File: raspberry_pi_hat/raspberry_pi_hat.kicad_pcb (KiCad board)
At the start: 2 copper layers, 100.5 x 49 mm, 18 parts, among them IC1 LD1117v33, J1 Screw_Terminal_01x02, J10 LED_status, J2 LCD_screeen, J8 GPIO, J9 Switches, U1 NRF24L01P

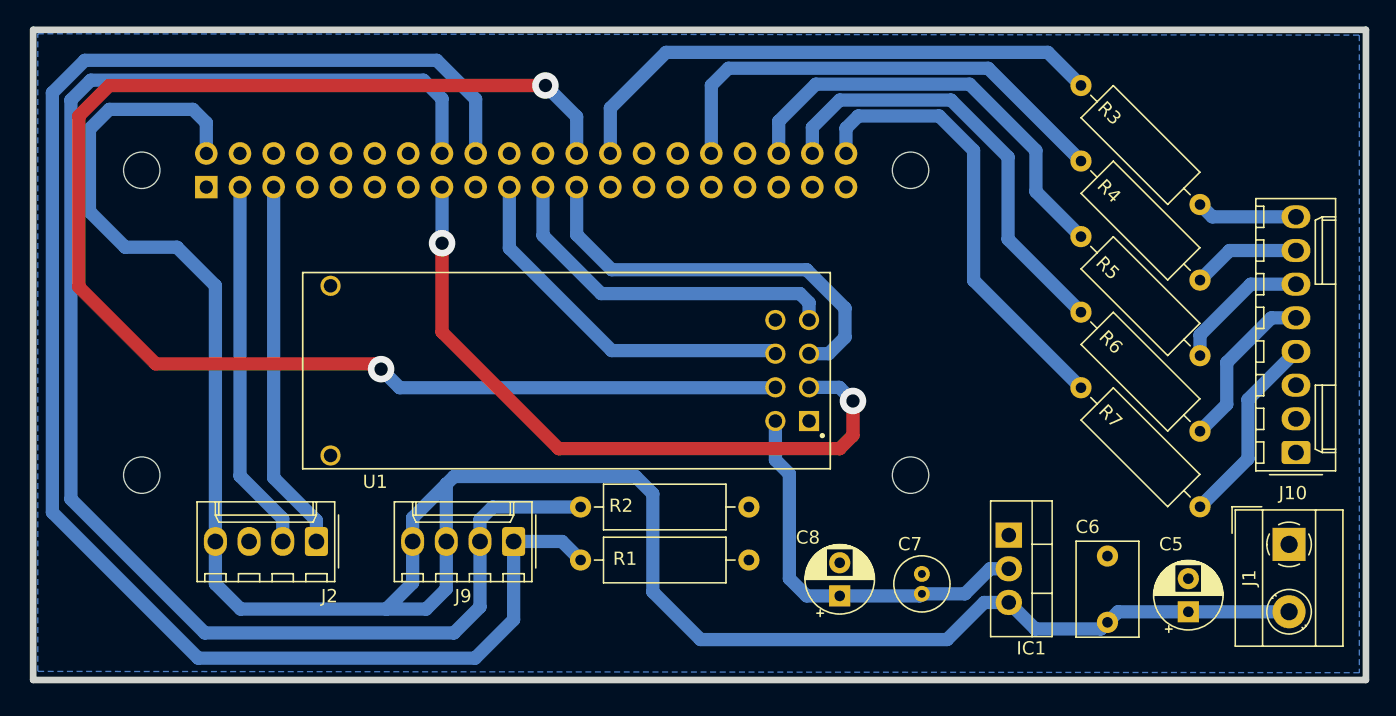
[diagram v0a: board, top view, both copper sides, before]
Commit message: improved final version
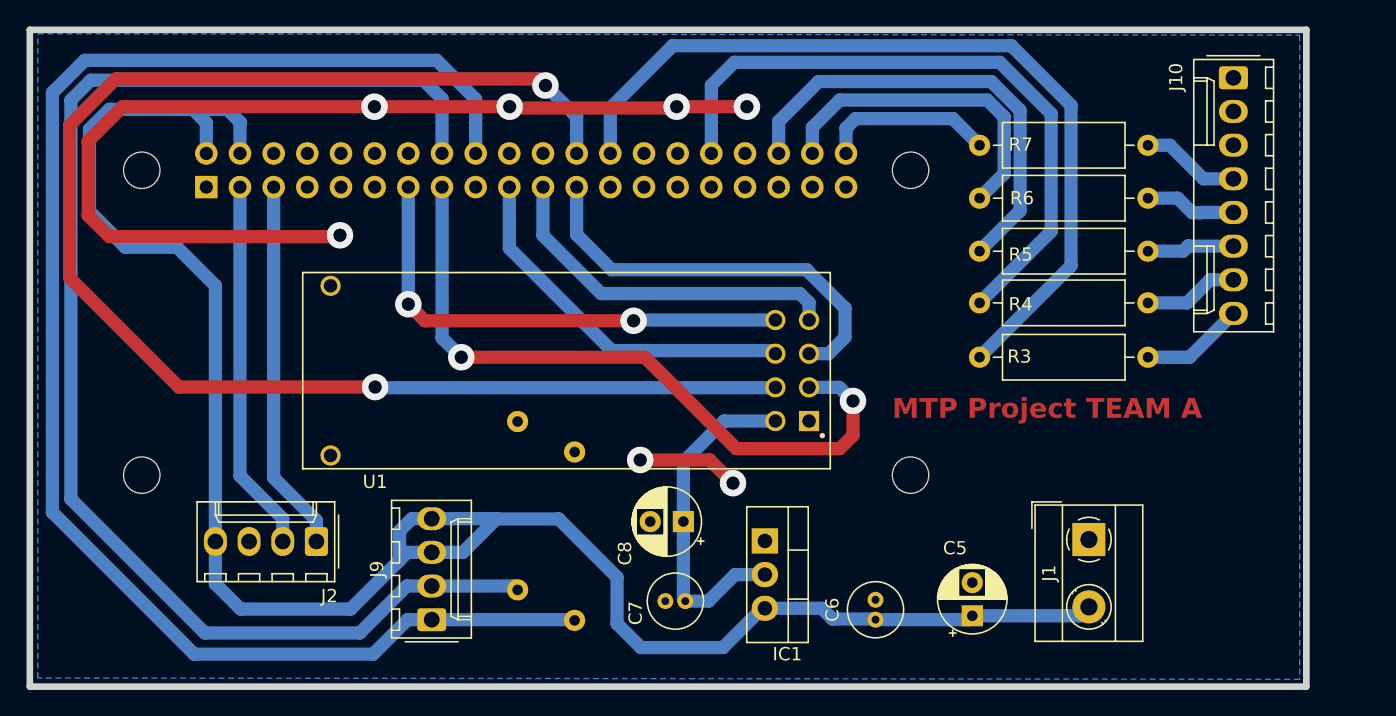
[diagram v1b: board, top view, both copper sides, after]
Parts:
- C6: footprint Capacitor_THT:C_Rect_L7.0mm_W4.5mm_P5.00mm -> Capacitor_THT:C_Radial_D4.0mm_H5.0mm_P1.50mm
- R1, R2: moved to B.Cu
- moved J10 28.7 mm to (205.5, 110.4), turned to -90 degrees
- moved R3 21.9 mm to (186.4, 131.5), turned to 0 degrees
- moved R7 19.8 mm to (186.4, 115.5), turned to 0 degrees
- moved IC1 18.4 mm to (170.2, 145.4)
- moved C7 17.9 mm to (164.2, 149.9), turned to 180 degrees
- moved C6 17.5 mm to (178.5, 151.3)
- moved C5 16.3 mm to (185.8, 151.0)
- moved J1 15.1 mm to (194.6, 145.3)
- moved R4 13.2 mm to (186.4, 127.4), turned to 0 degrees
- moved C8 13.1 mm to (164.0, 143.9), turned to 180 degrees
- moved R6 11.5 mm to (186.4, 119.5), turned to 0 degrees
- moved J9 8.54 mm to (145.0, 151.3), turned to 90 degrees
- moved R2 7.85 mm to (151.5, 149.1), turned to 90 degrees
- moved R5 7.73 mm to (186.4, 123.5), turned to 0 degrees
- moved R1 4.57 mm to (155.8, 151.3), turned to 90 degrees
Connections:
- U1 pad 8: unconnected-(U1-~{IRQ}-Pad8) -> /GPIO27
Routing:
- net GND: track 0.00 -> 83.9 mm, vias 0 -> 7
- net /GPIO27: track 0.00 -> 37.1 mm, vias 0 -> 2
- net /GPIO7/SPI0.CE1: track 41.7 -> 63.8 mm
- net /GPIO21/PCM.DOUT: track 34.2 -> 13.1 mm
- net +5V: track 166.5 -> 146.7 mm
- net /GPIO12/PWM0: track 36.6 -> 49.6 mm
- net /GPIO23: track 113.9 -> 102.9 mm
- net /GPIO20/PCM.DIN: track 33.3 -> 24.7 mm
- net Net-(J10-Pin_4): track 14.7 -> 7.50 mm
- net /GPIO24: track 122.0 -> 114.8 mm
- net Net-(J10-Pin_5): track 12.6 -> 6.91 mm
- net +3V3: track 30.3 -> 25.6 mm
- net Net-(J10-Pin_6): track 10.4 -> 6.62 mm
- net /GPIO16: track 33.0 -> 34.7 mm
- net CSN: track 110.9 -> 111.9 mm
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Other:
- board size 100.5 x 49 mm -> 96.3 x 49.5 mm
- board text added: "MTP Project TEAM A"
